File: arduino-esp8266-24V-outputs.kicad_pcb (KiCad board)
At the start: 2 copper layers, 99.7 x 99.7 mm, 47 parts, among them J1 Conn_01x02_Female, J2 Conn_01x02_Female, J3 Conn_01x02_Female, J4 Conn_01x02_Female, J5 Conn_01x02_Female, J6 Conn_01x02_Female, U1 WeMos_mini, U10 PC817, U11 PC817, U2 PC817, U3 PC817, U4 PC817, U5 PC817, U6 PC817, U7 PC817, U8 PC817, U9 PC817

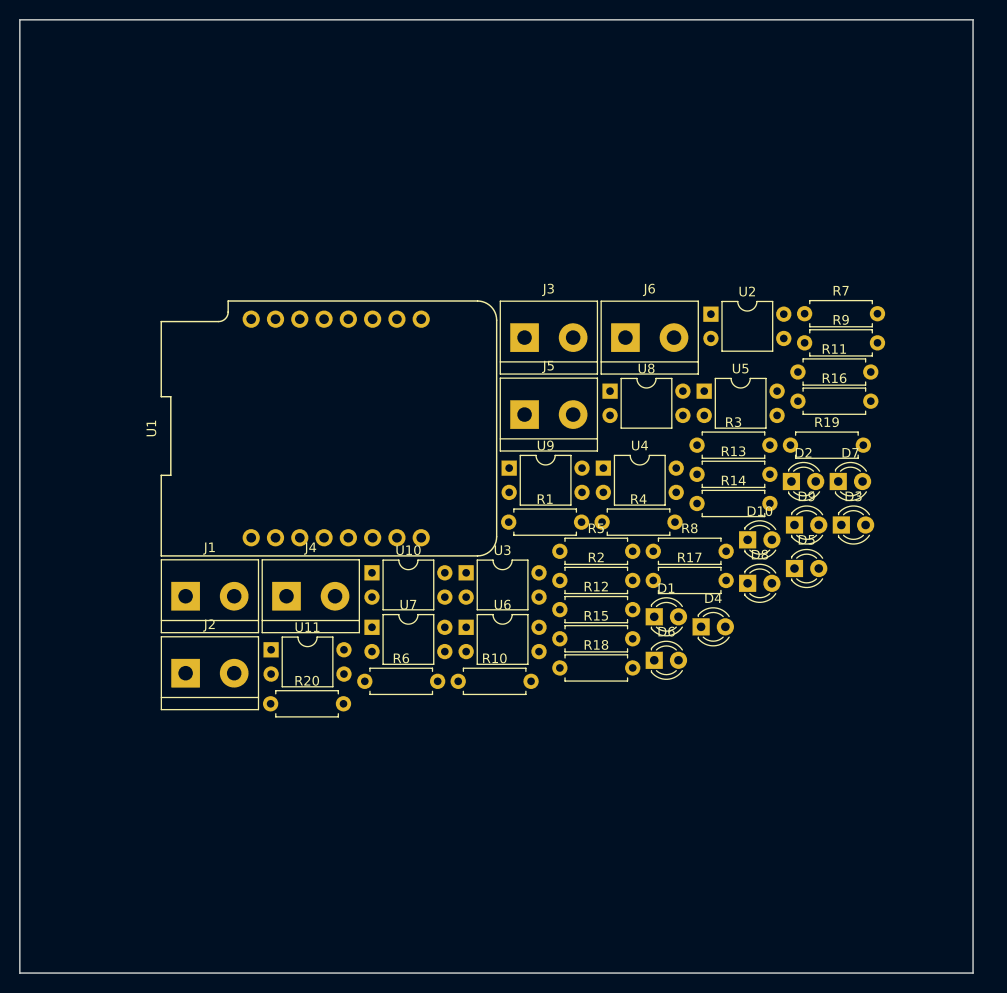
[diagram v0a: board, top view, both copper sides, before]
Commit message: finish tracks and layout
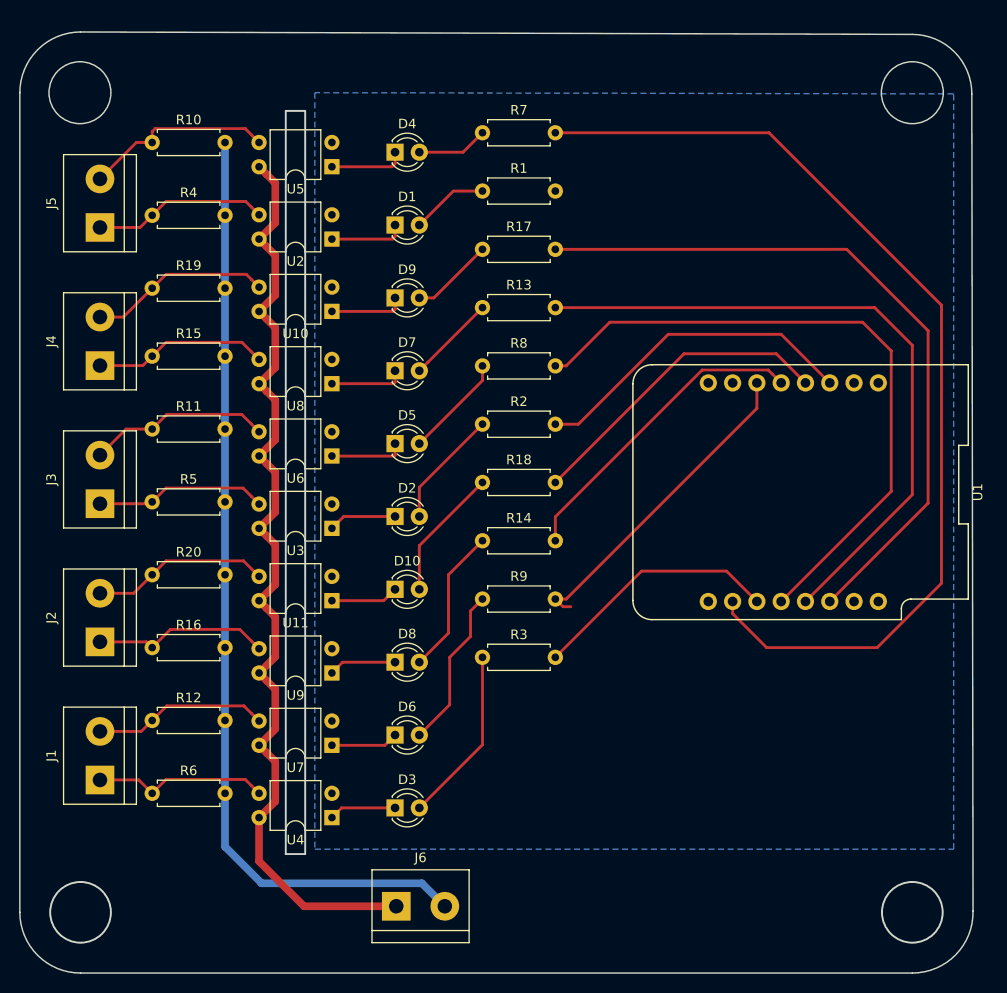
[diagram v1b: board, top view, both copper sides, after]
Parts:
- moved R16 72.3 mm to (28.4, 161.5)
- moved R19 68.7 mm to (28.4, 124.0)
- moved R11 67.8 mm to (28.4, 138.7)
- moved R10 64.8 mm to (28.4, 108.7)
- moved J6 64.1 mm to (54.0, 188.6)
- moved D4 59.1 mm to (53.8, 109.7)
- moved R4 57.0 mm to (28.4, 116.3)
- moved D3 55.3 mm to (53.8, 178.3)
- moved R15 51.9 mm to (28.4, 131.1)
- moved D1 49.1 mm to (53.8, 117.3)
- moved J5 48.5 mm to (23.0, 117.6), turned to 90 degrees
- moved U1 48.3 mm to (95.5, 145.3), turned to 180 degrees
- moved D9 48.1 mm to (53.8, 125.0)
- moved D7 47.8 mm to (53.8, 132.6)
- moved J3 47.7 mm to (23.0, 146.5), turned to 90 degrees
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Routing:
- net /D9: track 0.00 -> 104.3 mm
- net /24V: track 0.00 -> 101.6 mm
- net /GNDout: track 0.00 -> 99.2 mm
- net /D7: track 0.00 -> 75.1 mm
- net /D6: track 0.00 -> 70.4 mm
- net /D5: track 0.00 -> 69.2 mm
- net /D4: track 0.00 -> 34.7 mm
- net /D1: track 0.00 -> 33.9 mm
- net /D2: track 0.00 -> 33.0 mm
- net /D3: track 0.00 -> 33.0 mm
- net /D0: track 0.00 -> 26.1 mm
- net /I0.9: track 0.00 -> 20.1 mm
- net /I0.5: track 0.00 -> 19.1 mm
- net /I0.7: track 0.00 -> 19.0 mm
- net /I0.3: track 0.00 -> 18.7 mm
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- added copper zone on B.Cu, net GND
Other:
- board size 99.7 x 99.7 mm -> 99.7 x 98.4 mm
- net class Default: clearance 0.2 -> 0.3; trace_width 0.25 -> 0.3
- net class power added: clearance 0.5, trace_width 0.8, via_dia 1, via_drill 0.5
- rule trace_clearance: 0.2 -> 0.3
- rule trace_min: 0.2 -> 0.3
